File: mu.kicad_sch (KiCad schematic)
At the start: 74 parts, among them J1 USB_C_Receptacle_USB2.0_16P, J2 Conn_02x03_Odd_Even, J3 Conn_02x03_Odd_Even, J4 2060-1452/998-404, J5 ESQ-110-X-X-D, U1 STM32F042F6P6, U10 TLV3603QDCKRQ1, U11 SN74LVC1G74DCUT, U12 LM4040AIM3-2.5/NOPB, U13 MCP4921-E/SN, U14 BMP390, U2 MAX5026EUT_T, U3 MICROFC-60035-SMT-TR1, U4 TLV70433DBVT, U5 W25Q128JVS, U6 OPA656NB/250, U7 USBLC6-2SC6, U8 LT3045xDD, U9 sn65hvd230

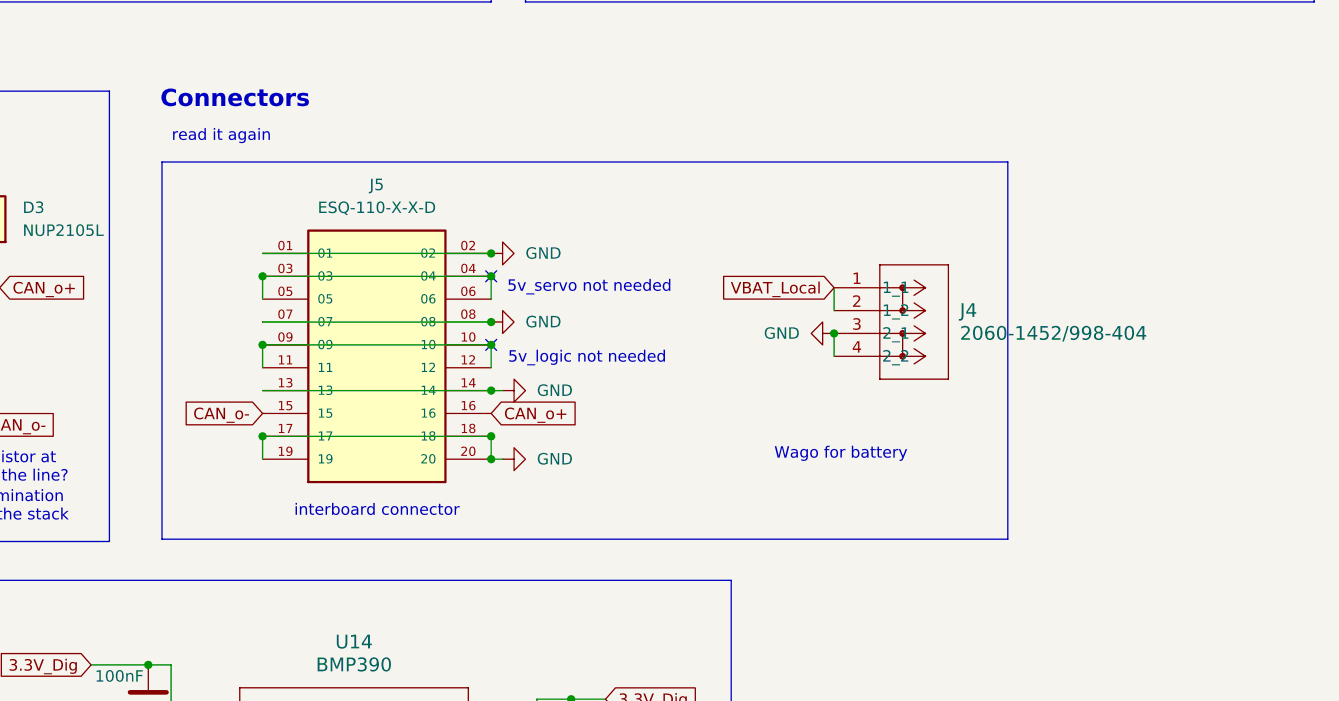
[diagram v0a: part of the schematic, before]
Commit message: ready to rock and roll
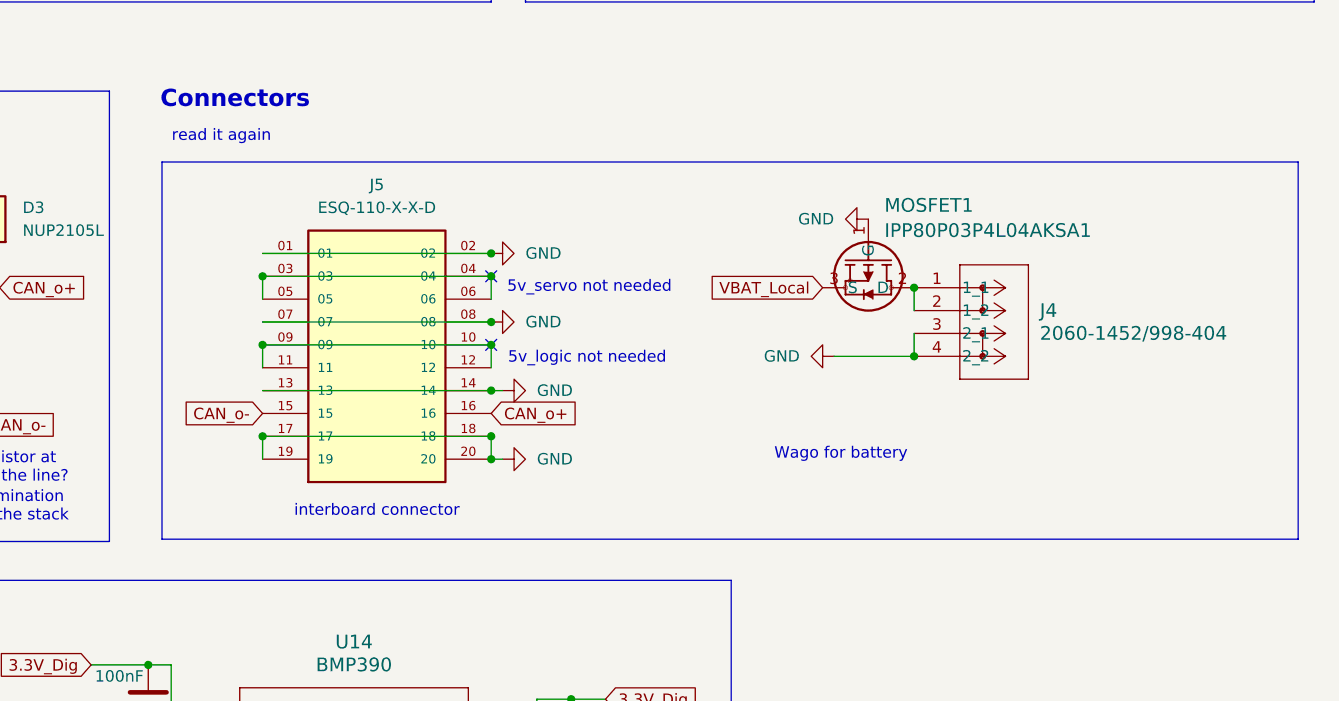
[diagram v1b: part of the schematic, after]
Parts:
- added MOSFET1: IPP80P03P4L04AKSA1, PG-TO220-3-1_INF, symbol IPP80P03P4L04AKSA1:IPP80P03P4L04AKSA1
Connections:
- net GND: now also MOSFET1.1 (G)
- net VBAT_Local: now also MOSFET1.3 (S); no longer J4.1 (1_1), J4.2 (1_2)
- new net: J4.1 (1_1), J4.2 (1_2), MOSFET1.2 (D)
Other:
- moved on the sheet: J4
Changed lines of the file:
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@@
 	(rectangle
 		(start 273.304 162.56)
-		(end 367.284 204.47)
+		(end 399.542 204.47)
 		(stroke
 			(width 0)
@@
 	)
 	(junction
+		(at 356.87 176.53)
+		(diameter 0)
+		(color 0 0 0 0)
+	)
+	(junction
 		(at 256.54 110.49)
 		(diameter 0)
@@
 	)
 	(junction
+		(at 356.87 184.15)
+		(diameter 0)
+		(color 0 0 0 0)
+	)
+	(junction
 		(at 172.72 238.76)
 		(diameter 0)
@@
 	)
 	(junction
-		(at 347.98 181.61)
-		(diameter 0)
-		(color 0 0 0 0)
-	)
-	(junction
 		(at 212.09 167.64)
 		(diameter 0)
@@
 	(wire
 		(pts
+			(xy 347.98 184.15) (xy 356.87 184.15)
+		)
+		(stroke
+			(width 0)
+			(type default)
+		)
+	)
+	(wire
+		(pts
 			(xy 231.14 181.61) (xy 231.14 191.77)
 		)
@@
 	(wire
 		(pts
+			(xy 356.87 176.53) (xy 356.87 179.07)
+		)
+		(stroke
+			(width 0)
+			(type default)
+		)
+	)
+	(wire
+		(pts
 			(xy 224.79 215.9) (xy 224.79 220.98)
 		)
@@
 	(wire
 		(pts
-			(xy 347.98 181.61) (xy 347.98 184.15)
-		)
-		(stroke
-			(width 0)
-			(type default)
-		)
-	)
-	(wire
-		(pts
 			(xy 205.74 73.66) (xy 203.2 73.66)
 		)
@@
 	(wire
 		(pts
+			(xy 356.87 181.61) (xy 356.87 184.15)
+		)
+		(stroke
+			(width 0)
+			(type default)
+		)
+	)
+	(wire
+		(pts
 			(xy 76.2 119.38) (xy 76.2 110.49)
 		)
@@
 	(wire
 		(pts
-			(xy 347.98 176.53) (xy 347.98 179.07)
-		)
-		(stroke
-			(width 0)
-			(type default)
-		)
-	)
-	(wire
-		(pts
 			(xy 248.92 191.77) (xy 252.73 191.77)
 		)
@@
 	(global_label "VBAT_Local"
 		(shape input)
-		(at 347.98 176.53 180)
+		(at 346.71 176.53 180)
 		(fields_autoplaced yes)
 		(effects
@@
 		)
 		(property "Intersheetrefs" "${INTERSHEET_REFS}"
-			(at 334.5325 176.53 0)
+			(at 333.2625 176.53 0)
 			(effects
 				(font
@@
 	(symbol
 		(lib_id "power:GND")
-		(at 347.98 181.61 270)
+		(at 347.98 184.15 270)
 		(unit 1)
 		(exclude_from_sim no)
@@
 		(fields_autoplaced yes)
 		(property "Reference" "#PWR046"
-			(at 341.63 181.61 0)
+			(at 341.63 184.15 0)
 			(effects
 				(font
@@
 		)
 		(property "Value" "GND"
-			(at 344.17 181.6099 90)
+			(at 344.17 184.1499 90)
 			(effects
 				(font
@@
 		)
 		(property "Footprint" ""
-			(at 347.98 181.61 0)
+			(at 347.98 184.15 0)
 			(effects
 				(font
@@
 		)
 		(property "Datasheet" ""
-			(at 347.98 181.61 0)
+			(at 347.98 184.15 0)
 			(effects
 				(font
@@
 		)
 		(property "Description" "Power symbol creates a global label with name \"GND\" , ground"
-			(at 347.98 181.61 0)
+			(at 347.98 184.15 0)
 			(effects
 				(font
@@
 	)
 	(symbol
+		(lib_id "power:GND")
+		(at 351.79 168.91 270)
+		(unit 1)
+		(exclude_from_sim no)
+		(in_bom yes)
+		(on_board yes)
+		(dnp no)
+		(fields_autoplaced yes)
+		(property "Reference" "#PWR053"
+			(at 345.44 168.91 0)
+			(effects
+				(font
+					(size 1.27 1.27)
+				)
+				(hide yes)
+			)
+		)
+		(property "Value" "GND"
+			(at 347.98 168.9099 90)
+			(effects
+				(font
+					(size 1.27 1.27)
+				)
+				(justify right)
+			)
+		)
+		(property "Footprint" ""
+			(at 351.79 168.91 0)
+			(effects
+				(font
+					(size 1.27 1.27)
+				)
+				(hide yes)
+			)
+		)
+		(property "Datasheet" ""
+			(at 351.79 168.91 0)
+			(effects
+				(font
+					(size 1.27 1.27)
+				)
+				(hide yes)
+			)
+		)
+		(property "Description" "Power symbol creates a global label with name \"GND\" , ground"
+			(at 351.79 168.91 0)
+			(effects
+				(font
+					(size 1.27 1.27)
+				)
+				(hide yes)
+			)
+		)
+		(pin "1"
+		)
+		(instances
+			(project "mu"
+				(path "/0020f91a-50ae-478d-8303-55d8991d2d34"
+					(reference "#PWR053")
+					(unit 1)
+				)
+			)
+		)
+	)
+	(symbol
 		(lib_id "Device:R")
 		(at 99.06 43.18 270)
@@
 	)
 	(symbol
+		(lib_id "IPP80P03P4L04AKSA1:IPP80P03P4L04AKSA1")
+		(at 351.79 168.91 270)
+		(unit 1)
+		(exclude_from_sim no)
+		(in_bom yes)
+		(on_board yes)
+		(dnp no)
+		(property "Reference" "MOSFET1"
+			(at 353.568 167.386 90)
+			(effects
+				(font
+					(size 1.524 1.524)
+				)
+				(justify left)
+			)
+		)
+		(property "Value" "IPP80P03P4L04AKSA1"
+			(at 353.568 170.18 90)
+			(effects
+				(font
+					(size 1.524 1.524)
+				)
+				(justify left)
+			)
+		)
+		(property "Footprint" "PG-TO220-3-1_INF"
+			(at 351.79 168.91 0)
+			(effects
+				(font
+					(size 1.27 1.27)
+					(italic yes)
+				)
+				(hide yes)
+			)
+		)
+		(property "Datasheet" "https://www.infineon.com/dgdl/Infineon-I80P03P4L_04-DS-v01_01-en.pdf?fileId=db3a30431ddc9372011e07e95eb827d7"
+			(at 351.79 168.91 0)
+			(effects
+				(font
+					(size 1.27 1.27)
+					(italic yes)
+				)
+				(hide yes)
+			)
+		)
+		(property "Description" ""
+			(at 351.79 168.91 0)
+			(effects
+				(font
+					(size 1.27 1.27)
+				)
+				(hide yes)
+			)
+		)
+		(pin "3"
+		)
+		(pin "2"
+		)
+		(pin "1"
+		)
+		(instances
+			(project ""
+				(path "/0020f91a-50ae-478d-8303-55d8991d2d34"
+					(reference "MOSFET1")
+					(unit 1)
+				)
+			)
+		)
+	)
+	(symbol
 		(lib_id "power:GND")
 		(at 245.11 101.6 270)
@@
 	(symbol
 		(lib_id "Wago_2060-1452 998-404:2060-1452_998-404")
-		(at 347.98 176.53 0)
+		(at 356.87 176.53 0)
 		(unit 1)
 		(exclude_from_sim no)
@@
 		(fields_autoplaced yes)
 		(property "Reference" "J4"
-			(at 361.95 179.0699 0)
+			(at 370.84 179.0699 0)
 			(effects
 				(font
@@
 		)
 		(property "Value" "2060-1452/998-404"
-			(at 361.95 181.6099 0)
+			(at 370.84 181.6099 0)
 			(effects
 				(font
@@
 		)
 		(property "Footprint" "footprints:WAG"
-			(at 347.98 176.53 0)
+			(at 356.87 176.53 0)
 			(effects
 				(font
@@
 		)
 		(property "Datasheet" "2060-1452/998-404"
-			(at 347.98 176.53 0)
+			(at 356.87 176.53 0)
 			(effects
 				(font
@@
 		)
 		(property "Description" ""
-			(at 347.98 176.53 0)
+			(at 356.87 176.53 0)
 			(effects
 				(font
@@
 		)
 		(instances
-			(project ""
+			(project "mu"
 				(path "/0020f91a-50ae-478d-8303-55d8991d2d34"
 					(reference "J4")
